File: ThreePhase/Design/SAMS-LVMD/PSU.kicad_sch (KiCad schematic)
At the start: 20 parts, among them J2 POWER INPUT, Q2 55V/42A

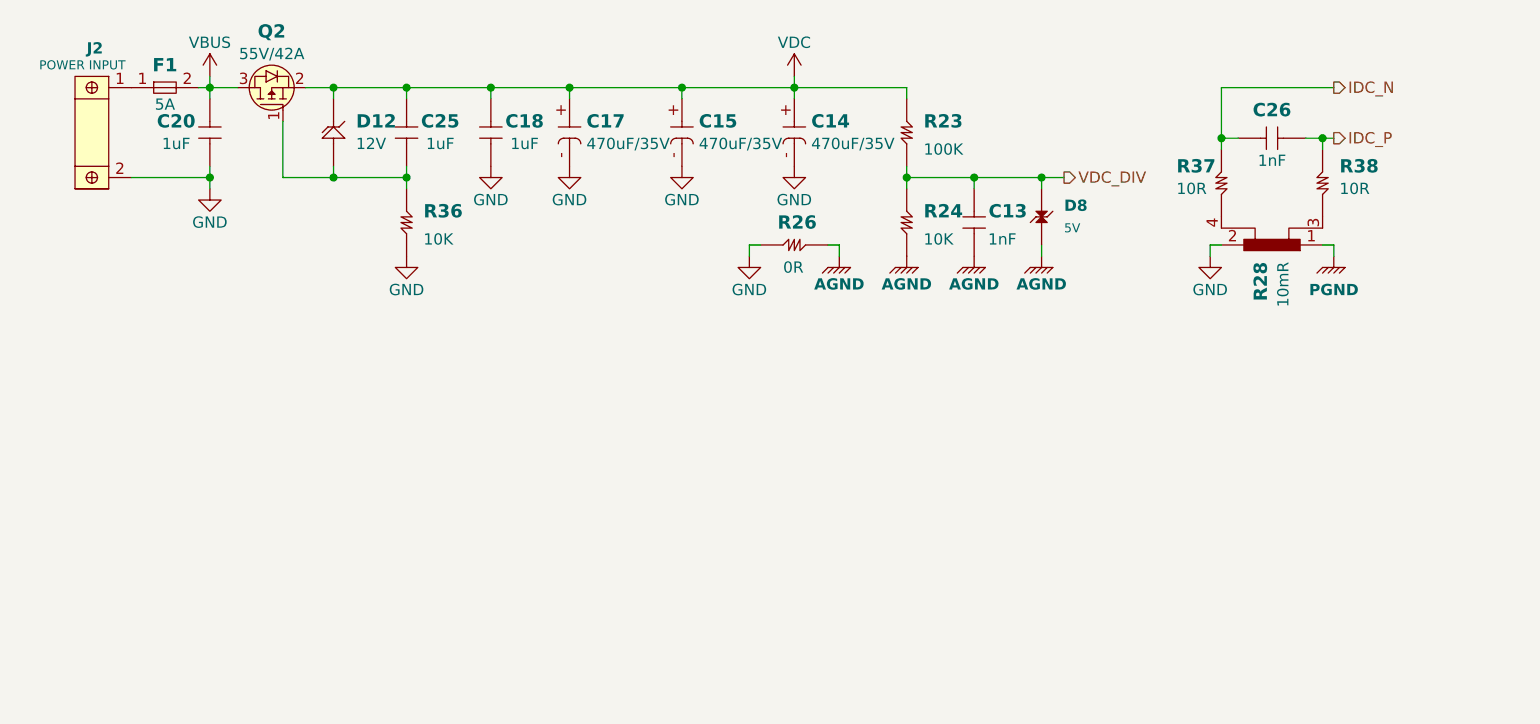
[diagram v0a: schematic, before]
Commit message: 3P schematic update 6
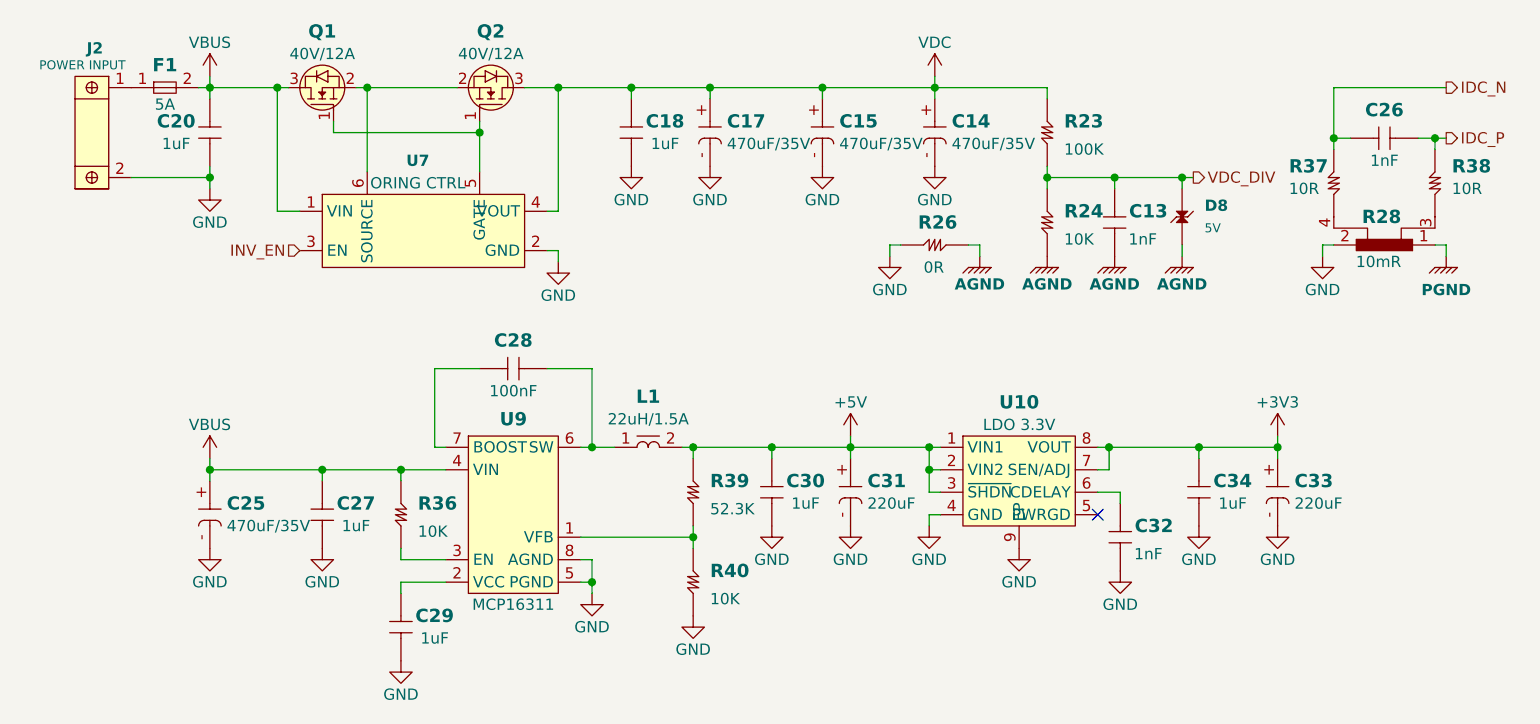
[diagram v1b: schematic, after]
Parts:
- removed C25: 1uF, SAMPI:CAP0603, symbol SAMPI:CERCAP
- removed D12: 12V, SAMPI:SOD-123, symbol Liem:DIODE-ZEN
- removed Q2: 55V/42A, SAMPI:D2PAK_TO-263, symbol Liem:FET_P-CH
- added C25: 470uF/35V, SAMPI:CAP_ELEC-10.3x10.3-DIA10, symbol SAMPI:ELECCAP
- added C27, C29, C30, C34: 1uF, SAMPI:CAP0603, symbol SAMPI:CERCAP
- added C28: 100nF, SAMPI:CAP0603, symbol SAMPI:CERCAP
- added C31, C33: 220uF, SAMPI:CAP_ELEC-10.3x10.3-DIA10, symbol SAMPI:ELECCAP
- added C32: 1nF, SAMPI:CAP0603, symbol SAMPI:CERCAP
- added L1: 22uH/1.5A, symbol SAMPI:IND
- added Q1, Q2: 40V/12A, SAMPI:D2PAK_TO-263, symbol Liem:FET_N-CH
- added R39: 52.3K, SAMPI:RES0603, symbol SAMPI:RES
- added R40: 10K, SAMPI:RES0603, symbol SAMPI:RES
- added U10: LDO 3.3V, symbol SAMPI:MCP1727
- added U7: ORING CTRL, SAMPI:SOT-23-6_MCHP, symbol SAMPI:KTS1900
- added U9: MCP16311, symbol SAMPI:MCP16311
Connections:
- net GND: now also C25.-, C27.1, C29.1, C30.1, C31.-, C32.1, C33.-, C34.1, R40.1, U10.4 (GND), U10.9 (EP), U7.2 (GND), U9.5 (PGND), U9.8 (AGND); no longer R36.1
- net VBUS: now also R36.2, C25.+, C27.2, Q1.3 (D), U7.1 (VIN), U9.4 (VIN)
- net VDC: now also Q2.3 (D), U7.4 (VOUT)
- new net: R39.1, R40.2, U9.1 (VFB)
- new net: Q1.1 (G), Q2.1 (G), U7.5 (GATE)
- new net: Q1.2 (S), Q2.2 (S), U7.6 (SOURCE)
- new net: C29.2, U9.2 (VCC)
- new net: C32.2, U10.6 (CDELAY)
- new net: R36.1, U9.3 (EN)
- new net: C28.1, L1.1, U9.6 (SW)
- new net: C28.2, U9.7 (BOOST)
- new net +3V3: C33.+, C34.2, U10.7 (SEN/ADJ), U10.8 (VOUT)
- new net +5V: C30.2, C31.+, L1.2, R39.2, U10.1 (VIN1), U10.2 (VIN2), U10.3 (~{SHDN})
- new net INV_EN: U7.3 (EN)
- no-connect marks 0 -> 1
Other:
- moved on the sheet: C13, C14, C15, C17, C18, C26, D8, R23, R24, R26, R28, R37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
